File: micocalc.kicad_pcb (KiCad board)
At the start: 2 copper layers, 58.4 x 78 mm, 41 parts, among them J1 Conn_01x02, J2 Conn_01x04, SW1 SW_Push_45deg, SW10 SW_Push_45deg, SW11 SW_Push_45deg, SW12 SW_Push_45deg, SW13 SW_Push_45deg, SW14 SW_Push_45deg, SW15 SW_Push_45deg, SW16 SW_Push_45deg, SW17 SW_SPST, SW18 SW_Push, SW2 SW_Push_45deg, SW3 SW_Push_45deg, SW4 SW_Push_45deg, SW5 SW_Push_45deg, SW6 SW_Push_45deg, SW7 SW_Push_45deg, SW8 SW_Push_45deg, SW9 SW_Push_45deg, U1 STM32L431RCTx, U2 HS96L03W2C03, U3 MCP1700x-120xxTT, Y1 8MHz

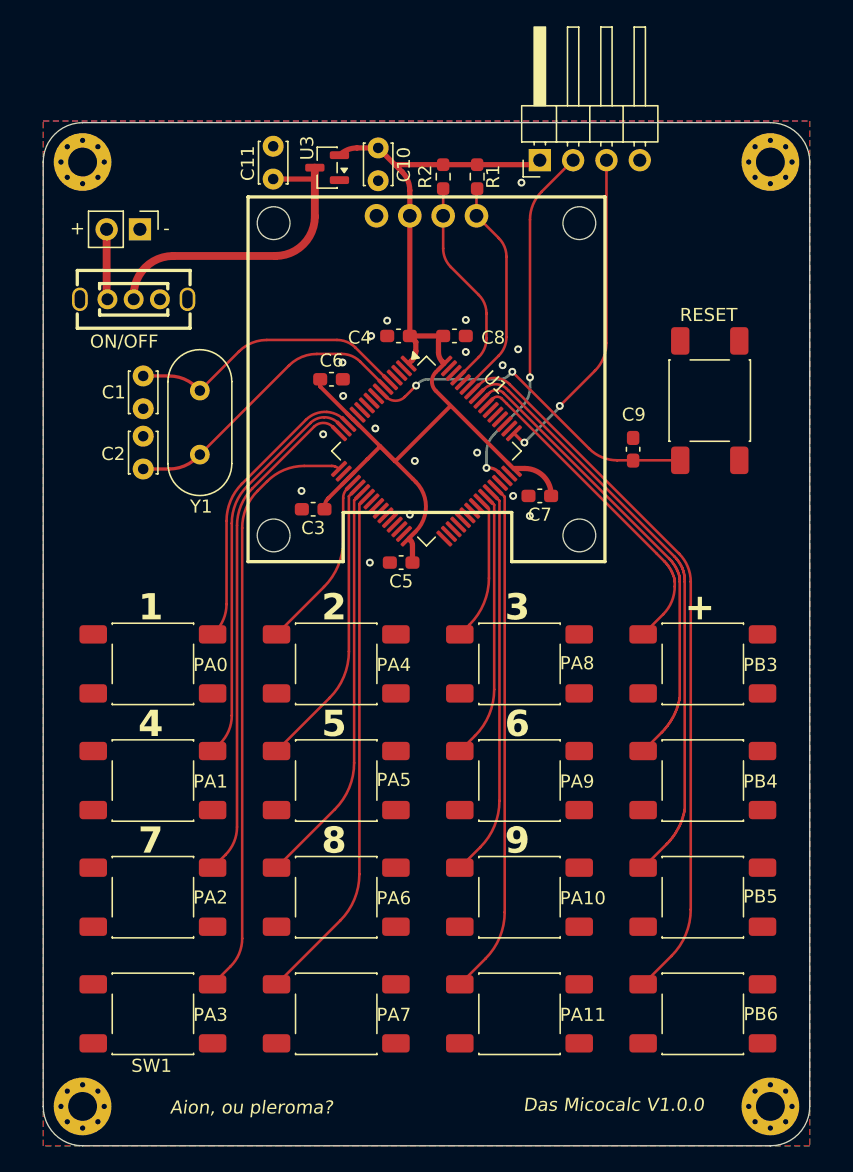
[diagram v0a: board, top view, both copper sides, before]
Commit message: improvements, better buttons
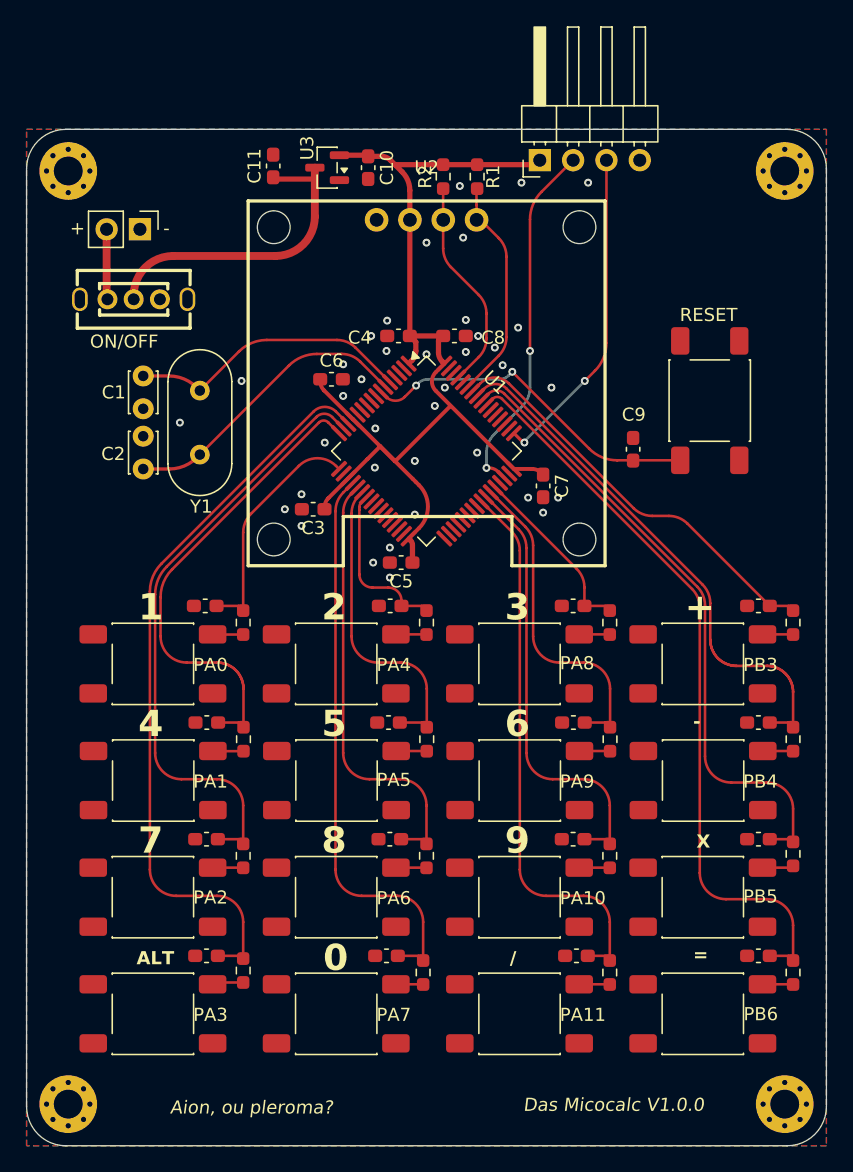
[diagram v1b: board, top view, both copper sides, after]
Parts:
- added C12: 1u, Capacitor_SMD:C_0603_1608Metric_Pad1.08x0.95mm_HandSolder, F.Cu at (110.1, 96.0)
- added C13: 1u, Capacitor_SMD:C_0603_1608Metric_Pad1.08x0.95mm_HandSolder, F.Cu at (110.3, 104.9)
- added C14: 1u, Capacitor_SMD:C_0603_1608Metric_Pad1.08x0.95mm_HandSolder, F.Cu at (110.2, 113.8)
- added C15: 1u, Capacitor_SMD:C_0603_1608Metric_Pad1.08x0.95mm_HandSolder, F.Cu at (110.2, 122.7)
- added C16: 1u, Capacitor_SMD:C_0603_1608Metric_Pad1.08x0.95mm_HandSolder, F.Cu at (124.2, 96.0)
- added C17: 1u, Capacitor_SMD:C_0603_1608Metric_Pad1.08x0.95mm_HandSolder, F.Cu at (124.1, 104.9)
- added C18: 1u, Capacitor_SMD:C_0603_1608Metric_Pad1.08x0.95mm_HandSolder, F.Cu at (124.2, 113.8)
- added C19: 1u, Capacitor_SMD:C_0603_1608Metric_Pad1.08x0.95mm_HandSolder, F.Cu at (124.0, 122.7)
- added C20: 1u, Capacitor_SMD:C_0603_1608Metric_Pad1.08x0.95mm_HandSolder, F.Cu at (138.2, 96.0)
- added C21: 1u, Capacitor_SMD:C_0603_1608Metric_Pad1.08x0.95mm_HandSolder, F.Cu at (138.2, 104.9)
- added C22: 1u, Capacitor_SMD:C_0603_1608Metric_Pad1.08x0.95mm_HandSolder, F.Cu at (138.2, 113.8)
- added C23: 1u, Capacitor_SMD:C_0603_1608Metric_Pad1.08x0.95mm_HandSolder, F.Cu at (138.4, 122.7)
- added C24: 1u, Capacitor_SMD:C_0603_1608Metric_Pad1.08x0.95mm_HandSolder, F.Cu at (152.3, 96.0)
- added C25: 1u, Capacitor_SMD:C_0603_1608Metric_Pad1.08x0.95mm_HandSolder, F.Cu at (152.3, 104.9)
- added C26: 1u, Capacitor_SMD:C_0603_1608Metric_Pad1.08x0.95mm_HandSolder, F.Cu at (152.3, 113.8)
- added C27: 1u, Capacitor_SMD:C_0603_1608Metric_Pad1.08x0.95mm_HandSolder, F.Cu at (152.3, 122.7)
- added R10: 2.2k, Resistor_SMD:R_0603_1608Metric_Pad0.98x0.95mm_HandSolder, F.Cu at (126.7, 124.0)
- added R11: 2.2k, Resistor_SMD:R_0603_1608Metric_Pad0.98x0.95mm_HandSolder, F.Cu at (141.0, 97.3)
- added R12: 2.2k, Resistor_SMD:R_0603_1608Metric_Pad0.98x0.95mm_HandSolder, F.Cu at (141.0, 106.2)
- added R13: 2.2k, Resistor_SMD:R_0603_1608Metric_Pad0.98x0.95mm_HandSolder, F.Cu at (141.0, 115.1)
- added R14: 2.2k, Resistor_SMD:R_0603_1608Metric_Pad0.98x0.95mm_HandSolder, F.Cu at (141.0, 124.0)
- added R15: 2.2k, Resistor_SMD:R_0603_1608Metric_Pad0.98x0.95mm_HandSolder, F.Cu at (154.9, 97.3)
- added R16: 2.2k, Resistor_SMD:R_0603_1608Metric_Pad0.98x0.95mm_HandSolder, F.Cu at (154.9, 106.2)
- added R17: 2.2k, Resistor_SMD:R_0603_1608Metric_Pad0.98x0.95mm_HandSolder, F.Cu at (154.9, 114.9)
- added R18: 2.2k, Resistor_SMD:R_0603_1608Metric_Pad0.98x0.95mm_HandSolder, F.Cu at (154.9, 124.0)
- added R3: 2.2k, Resistor_SMD:R_0603_1608Metric_Pad0.98x0.95mm_HandSolder, F.Cu at (113.0, 97.3)
- added R4: 2.2k, Resistor_SMD:R_0603_1608Metric_Pad0.98x0.95mm_HandSolder, F.Cu at (113.1, 106.2)
- added R5: 2.2k, Resistor_SMD:R_0603_1608Metric_Pad0.98x0.95mm_HandSolder, F.Cu at (113.0, 115.1)
- added R6: 2.2k, Resistor_SMD:R_0603_1608Metric_Pad0.98x0.95mm_HandSolder, F.Cu at (113.0, 123.8)
- added R7: 2.2k, Resistor_SMD:R_0603_1608Metric_Pad0.98x0.95mm_HandSolder, F.Cu at (127.0, 97.3)
- added R8: 2.2k, Resistor_SMD:R_0603_1608Metric_Pad0.98x0.95mm_HandSolder, F.Cu at (127.0, 106.2)
- added R9: 2.2k, Resistor_SMD:R_0603_1608Metric_Pad0.98x0.95mm_HandSolder, F.Cu at (127.0, 115.1)
- C10, C11: footprint Capacitor_THT:C_Disc_D3.0mm_W2.0mm_P2.50mm -> Capacitor_SMD:C_0603_1608Metric_Pad1.08x0.95mm_HandSolder
- C3, C4, C5, C6, C7, C8, C9: value 0.1u -> 1u
- moved SW1 26.7 mm to (106.2, 100.4)
- moved SW12 26.7 mm to (134.1, 127.1)
- moved SW13 26.7 mm to (148.1, 100.4)
- moved SW16 26.7 mm to (148.1, 127.1)
- moved SW4 26.7 mm to (106.2, 127.1)
- moved SW5 26.7 mm to (120.1, 100.4)
- moved SW8 26.7 mm to (120.1, 127.1)
- moved SW9 26.7 mm to (134.1, 100.4)
- moved SW10 8.89 mm to (134.1, 109.3)
- moved SW14 8.89 mm to (148.1, 109.3)
- moved SW2 8.89 mm to (106.2, 109.3)
- moved SW6 8.89 mm to (120.1, 109.3)
- moved SW11 8.89 mm to (134.1, 118.2)
- moved SW15 8.89 mm to (148.1, 118.2)
- moved SW3 8.89 mm to (106.2, 118.2)
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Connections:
- SW1 pad 1: Net-(U1-PA3) -> Net-(R3-Pad2)
- SW10 pad 1: Net-(U1-PA10) -> Net-(R12-Pad2)
- SW11 pad 1: Net-(U1-PA9) -> Net-(R13-Pad2)
- SW12 pad 1: Net-(U1-PA8) -> Net-(R14-Pad2)
- SW13 pad 1: Net-(U1-PB6) -> Net-(R15-Pad2)
- SW14 pad 1: Net-(U1-PB5) -> Net-(R16-Pad2)
- SW15 pad 1: Net-(U1-PB4) -> Net-(R17-Pad2)
- SW16 pad 1: Net-(U1-PB3) -> Net-(R18-Pad2)
- SW2 pad 1: Net-(U1-PA2) -> Net-(R4-Pad2)
- SW3 pad 1: Net-(U1-PA1) -> Net-(R5-Pad2)
- SW4 pad 1: Net-(U1-PA0) -> Net-(R6-Pad2)
- SW5 pad 1: Net-(U1-PA7) -> Net-(R7-Pad2)
- SW6 pad 1: Net-(U1-PA6) -> Net-(R8-Pad2)
- SW7 pad 1: Net-(U1-PA5) -> Net-(R9-Pad2)
- SW8 pad 1: Net-(U1-PA4) -> Net-(R10-Pad2)
- SW9 pad 1: Net-(U1-PA11) -> Net-(R11-Pad2)
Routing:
- net Net-(U1-PA0): track 22.6 -> 57.1 mm
- net Net-(U1-PB3): track 25.6 -> 57.6 mm
- net Net-(U1-PA8): track 11.0 -> 42.9 mm
- net Net-(U1-PA4): track 13.7 -> 43.7 mm
- net Net-(U1-PA3): track 45.6 -> 18.4 mm
- net Net-(U1-PA7): track 39.8 -> 12.9 mm
- net Net-(U1-PA11): track 39.3 -> 13.8 mm
- net Net-(U1-PB6): track 55.8 -> 31.9 mm
- net Net-(U1-PA1): track 30.7 -> 46.9 mm
- net Net-(U1-PA9): track 20.5 -> 34.2 mm
- net Net-(U1-PB4): track 35.7 -> 49.2 mm
- net Net-(U1-PA5): track 22.4 -> 34.1 mm
- net Net-(U1-PA6): track 31.1 -> 24.2 mm
- net Net-(U1-PA10): track 29.9 -> 25.2 mm
- net Net-(U1-PB5): track 45.8 -> 41.3 mm
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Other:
- board size 58.4 x 78 mm -> 61 x 77.5 mm
- board text added: "/"
- board text added: "0"
- board text added: "="
- board text added: "ALT"
- board text added: "X"
- board text added: "https://github.com/hadron13/DasMicocalc"
